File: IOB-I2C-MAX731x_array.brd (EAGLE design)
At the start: 108.7 x 112 mm, 30 parts, among them IC1X11 MAX7311, IC1X12 MAX7311, IC1X13 MAX7311, SW1X11 A0, SW1X12 A0, SW1X13 A0, SW2X11 A1, SW2X12 A1, SW2X13 A1, SW3X11 A2, SW3X12 A2, SW3X13 A2

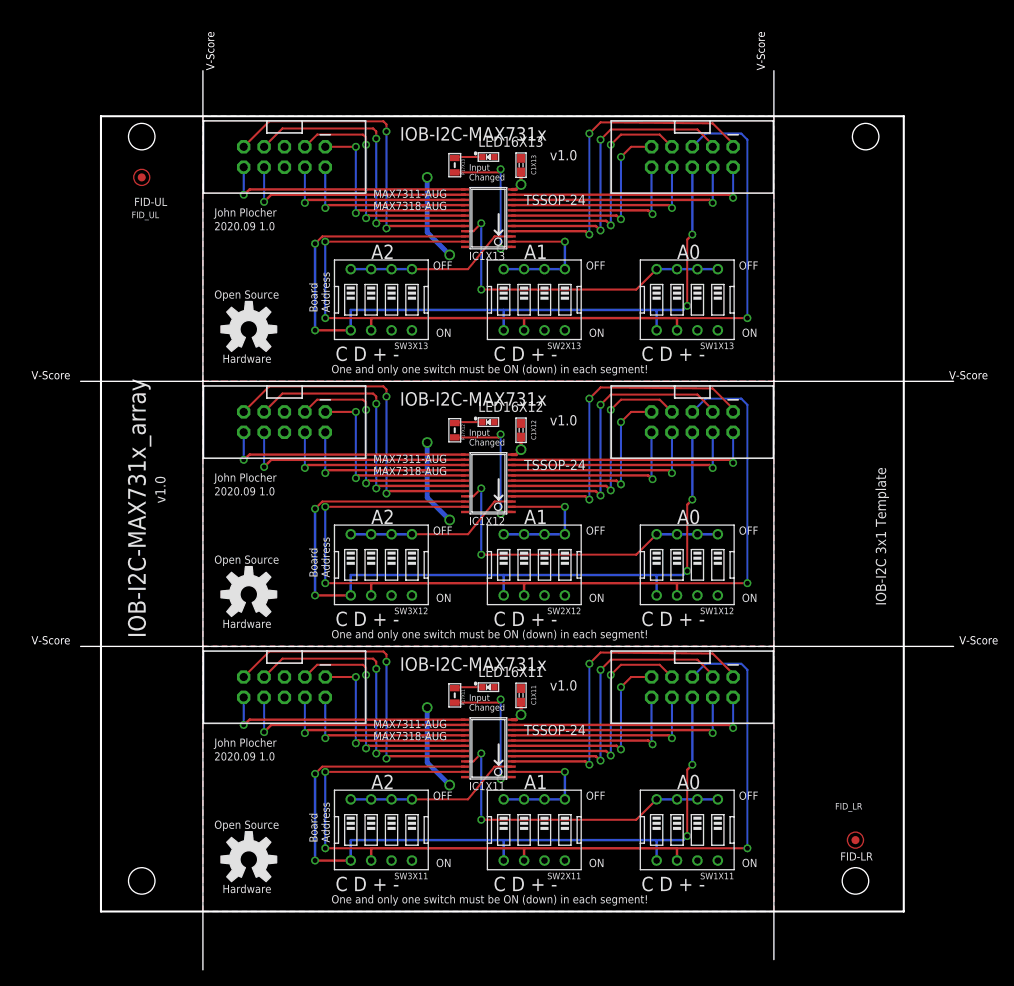
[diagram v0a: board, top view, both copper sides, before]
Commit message: cleanup layout
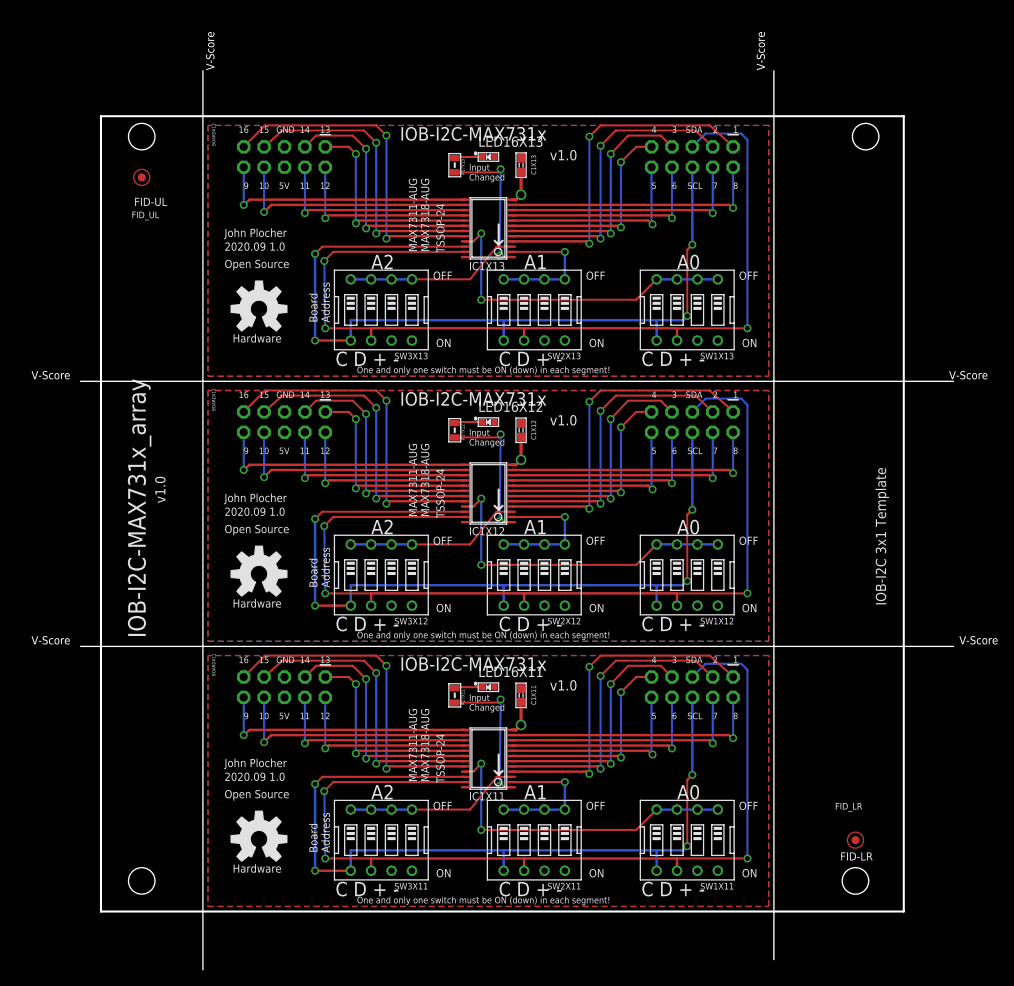
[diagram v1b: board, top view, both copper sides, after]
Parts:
- BOARDX11, BOARDX12, BOARDX13: value I2C-EXPANDER -> CONNECTOR-I2C-EXPANDER
- moved U$1X13 2.84 mm to (19.7, 75.1)
- moved U$1X11 2.84 mm to (19.7, 9.02)
- moved U$1X12 2.84 mm to (19.7, 42.0)
- moved IC1X12 1.27 mm to (48.3, 52.1)
- moved SW1X12 1.27 mm to (73.0, 41.9)
- moved SW2X12 1.27 mm to (54.0, 41.9)
- moved SW3X12 1.27 mm to (34.9, 41.9)
- moved IC1X11 1.27 mm to (48.3, 19.1)
- moved SW1X11 1.27 mm to (73.0, 8.89)
- moved SW2X11 1.27 mm to (54.0, 8.89)
- moved SW3X11 1.27 mm to (34.9, 8.89)
- moved IC1X13 1.27 mm to (48.3, 85.1)
- moved SW1X13 1.27 mm to (73.0, 74.9)
- moved SW2X13 1.27 mm to (54.0, 74.9)
- moved SW3X13 1.27 mm to (34.9, 74.9)
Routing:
- net VCCX13: track 10.8 -> 0.00 mm, vias 2 -> 0
- net VCCX12: track 10.8 -> 0.00 mm, vias 2 -> 0
- net VCCX11: track 10.8 -> 0.00 mm, vias 2 -> 0
- net P9X13: track 31.2 -> 32.5 mm
- net P8X13: track 31.5 -> 32.8 mm
- net P9X12: track 31.2 -> 32.5 mm
- net P7X11: track 29.6 -> 30.9 mm
- net P8X12: track 31.5 -> 32.8 mm
- net P11X11: track 24.5 -> 25.8 mm
- net P10X12: track 29.7 -> 31.0 mm
- net P8X11: track 31.5 -> 32.8 mm
- net P6X11: track 25.2 -> 26.4 mm
- net P5X11: track 23.7 -> 24.9 mm
- net P12X11: track 22.6 -> 23.9 mm
- net P10X11: track 29.7 -> 31.0 mm
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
